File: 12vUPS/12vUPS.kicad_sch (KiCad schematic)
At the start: 13 parts, among them J1 INPUT, J2 OUTPUT, J3 BATTERY, K1 VEGHA L08A0212VDC, Q1 BDX53C

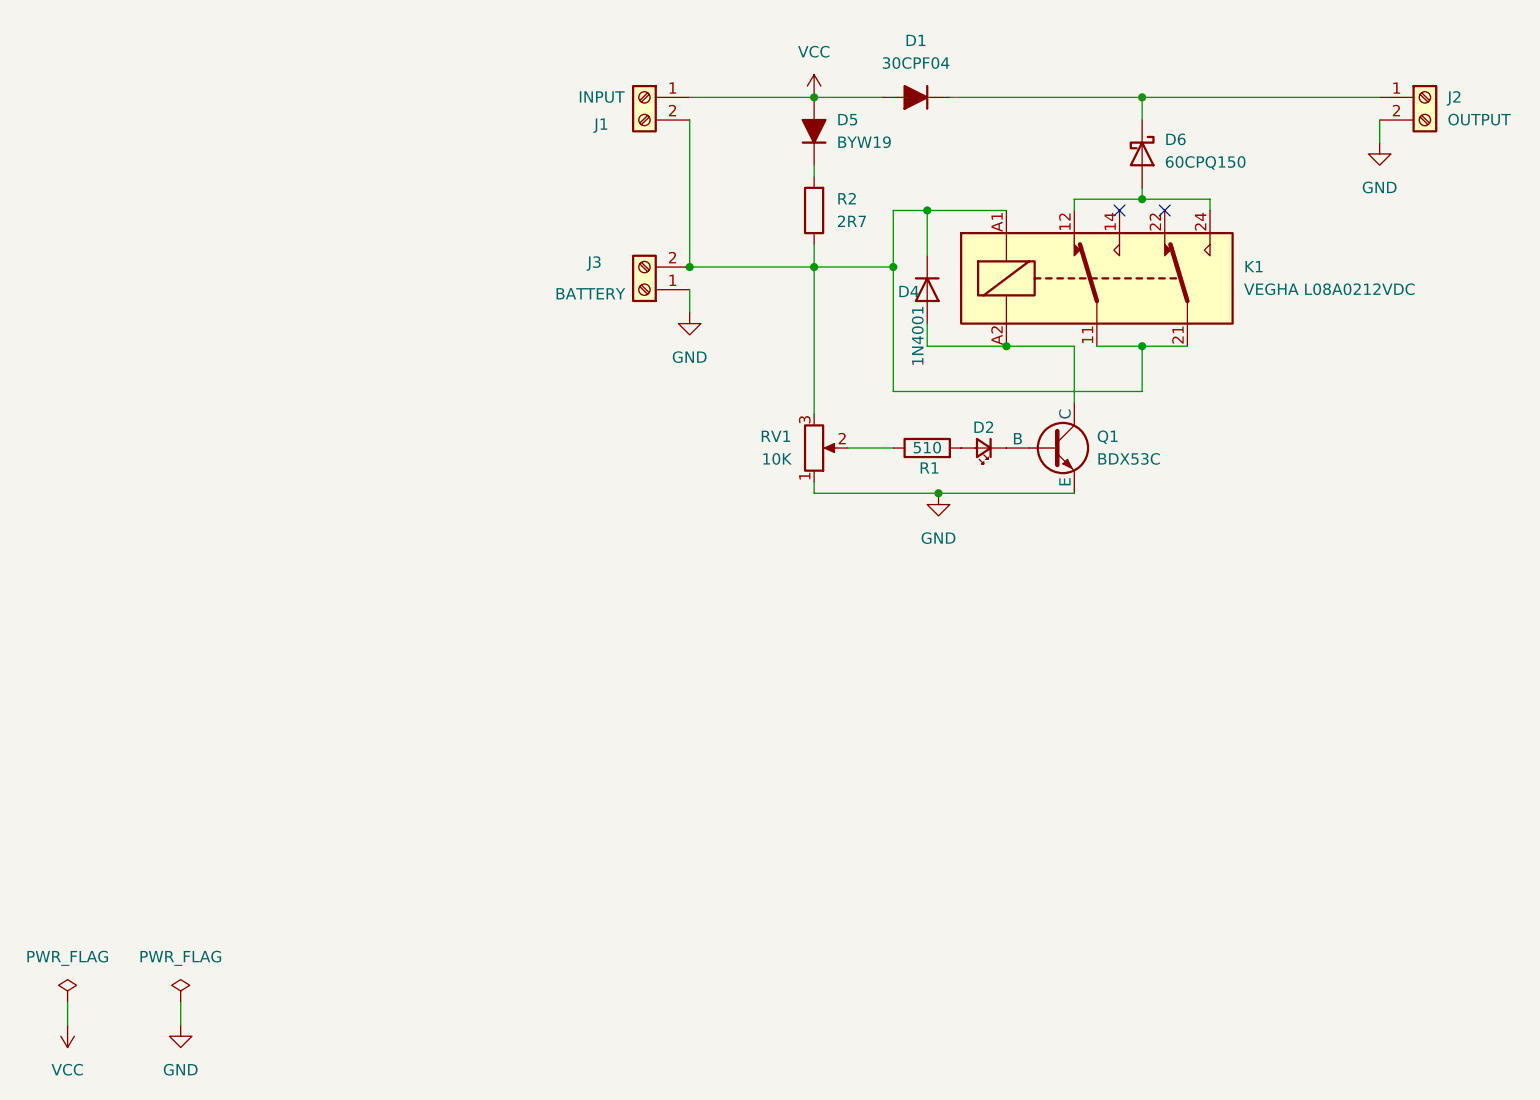
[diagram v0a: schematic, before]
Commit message: Update 12vUPS-2025-06-02_174418.zip, 12vUPS-2025-06-06_223532.zip, 12vUPS-2025-06-06_224038.zip, and 9 more files
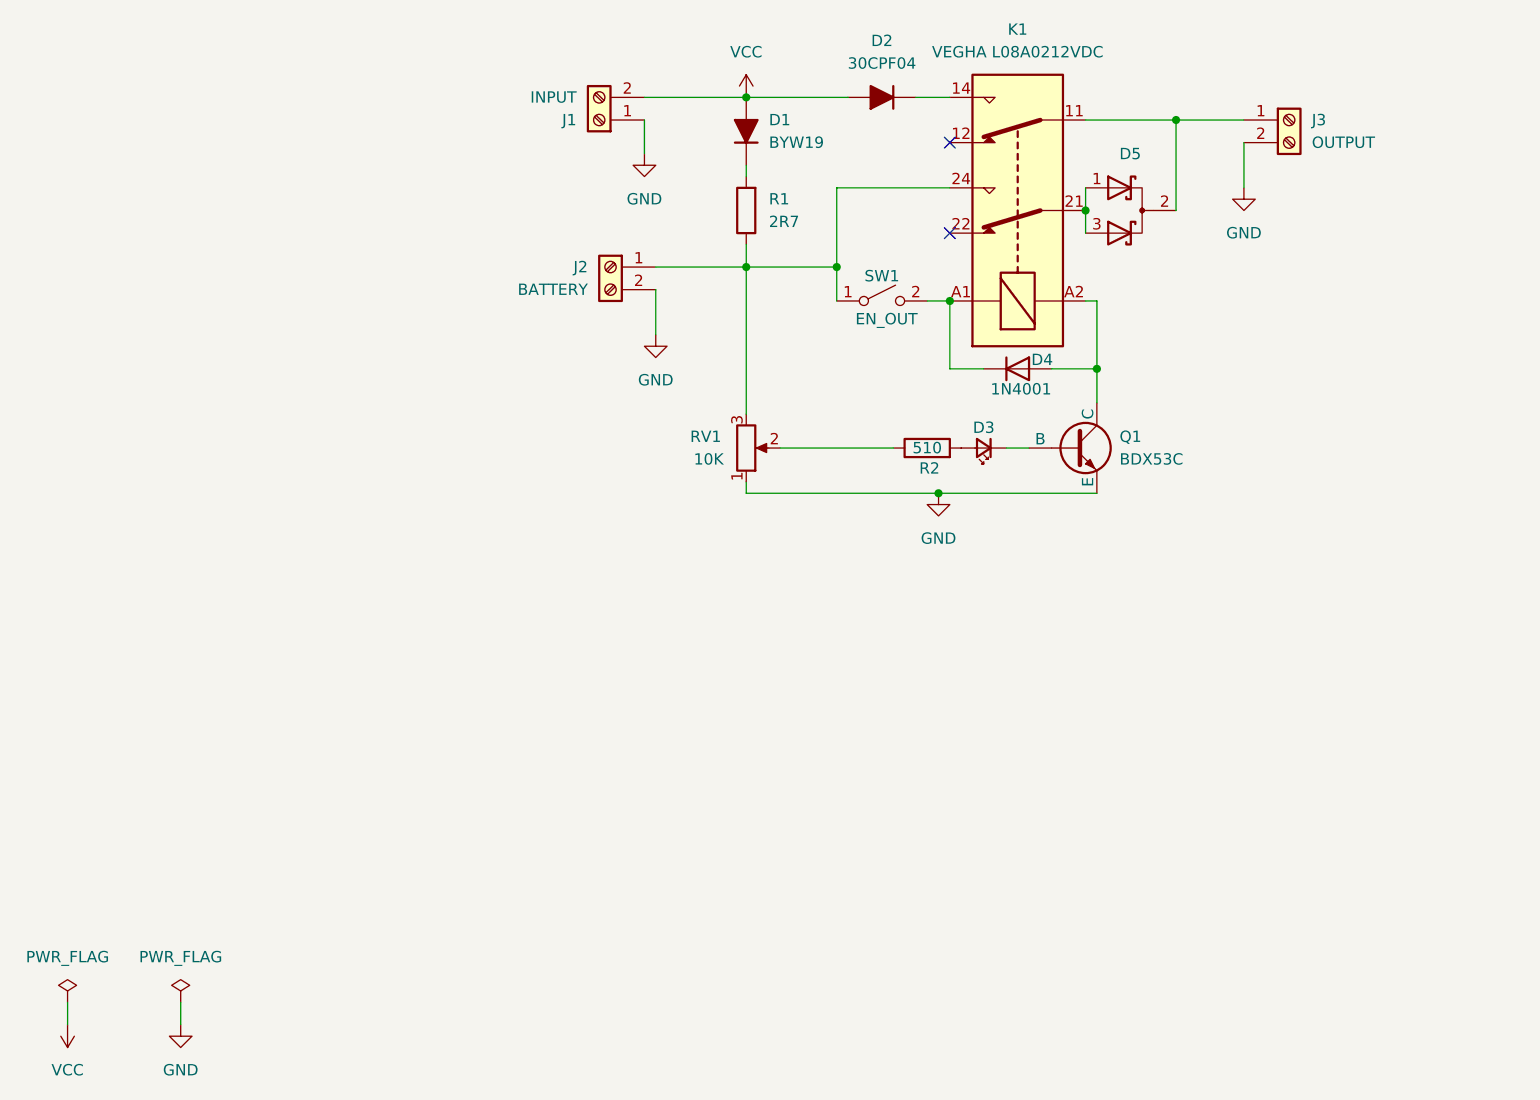
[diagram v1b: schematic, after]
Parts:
- removed D6: 60CPQ150, Package_TO_SOT_THT:TO-247-3_Vertical, symbol Device:D_Schottky
- removed J3: BATTERY, TerminalBlock:TerminalBlock_bornier-2_P5.08mm, symbol Connector:Screw_Terminal_01x02
- added D5: D_Schottky_Dual_CommonCathode_AKA_Parallel, Package_TO_SOT_THT:TO-247-3_Vertical, symbol Device:D_Schottky_Dual_CommonCathode_AKA_Parallel
- added J2: BATTERY, TerminalBlock_MetzConnect:TerminalBlock_MetzConnect_Type703_RT10N02HGLU_1x02_P9.52mm_Horizontal, symbol Connector:Screw_Terminal_01x02
- added SW1: EN_OUT, symbol Switch:SW_SPST
- J1: footprint TerminalBlock:TerminalBlock_bornier-2_P5.08mm -> TerminalBlock_MetzConnect:TerminalBlock_MetzConnect_Type703_RT10N02HGLU_1x02_P9.52mm_Horizontal
- J3: renamed from J2; footprint TerminalBlock:TerminalBlock_bornier-2_P5.08mm -> TerminalBlock_MetzConnect:TerminalBlock_MetzConnect_Type703_RT10N02HGLU_1x02_P9.52mm_Horizontal
- K1: footprint Relay_THT:Relay_SPDT_Schrack-RP-II-1-16A-FormC_RM5mm -> IK5PWC:VEGhA L08 12V dc
- RV1: footprint (none) -> Potentiometer_THT:Potentiometer_Vishay_T93YA_Vertical
- renumbered D5 to D1, D1 to D2, D2 to D3, R2 to R1, R1 to R2
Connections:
- net GND: now also J1.1 (Pin_1), J2.2 (Pin_2)
- net VCC: now also J1.2 (Pin_2); no longer J1.1 (Pin_1)
- net at D2.1 (K): now also K1.14; no longer J3.1 (Pin_1)
- net at K1.24: now also R1.1, RV1.3, J2.1 (Pin_1), SW1.1 (A); no longer K1.12
- new net: D5.2 (K), J3.1 (Pin_1), K1.11
- new net: D5.1 (A), D5.3 (A), K1.21
- new net: D4.1 (K), K1.A1, SW1.2 (B)
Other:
- moved on the sheet: D1, D2, D4, J3, K1, Q1, R1, RV1
